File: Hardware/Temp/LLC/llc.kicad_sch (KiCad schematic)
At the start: 23 parts, among them M1 650 V, 24 A, M2 650 V, 24 A, U1 IR2101, U2 OPAMP_OP07CSZ

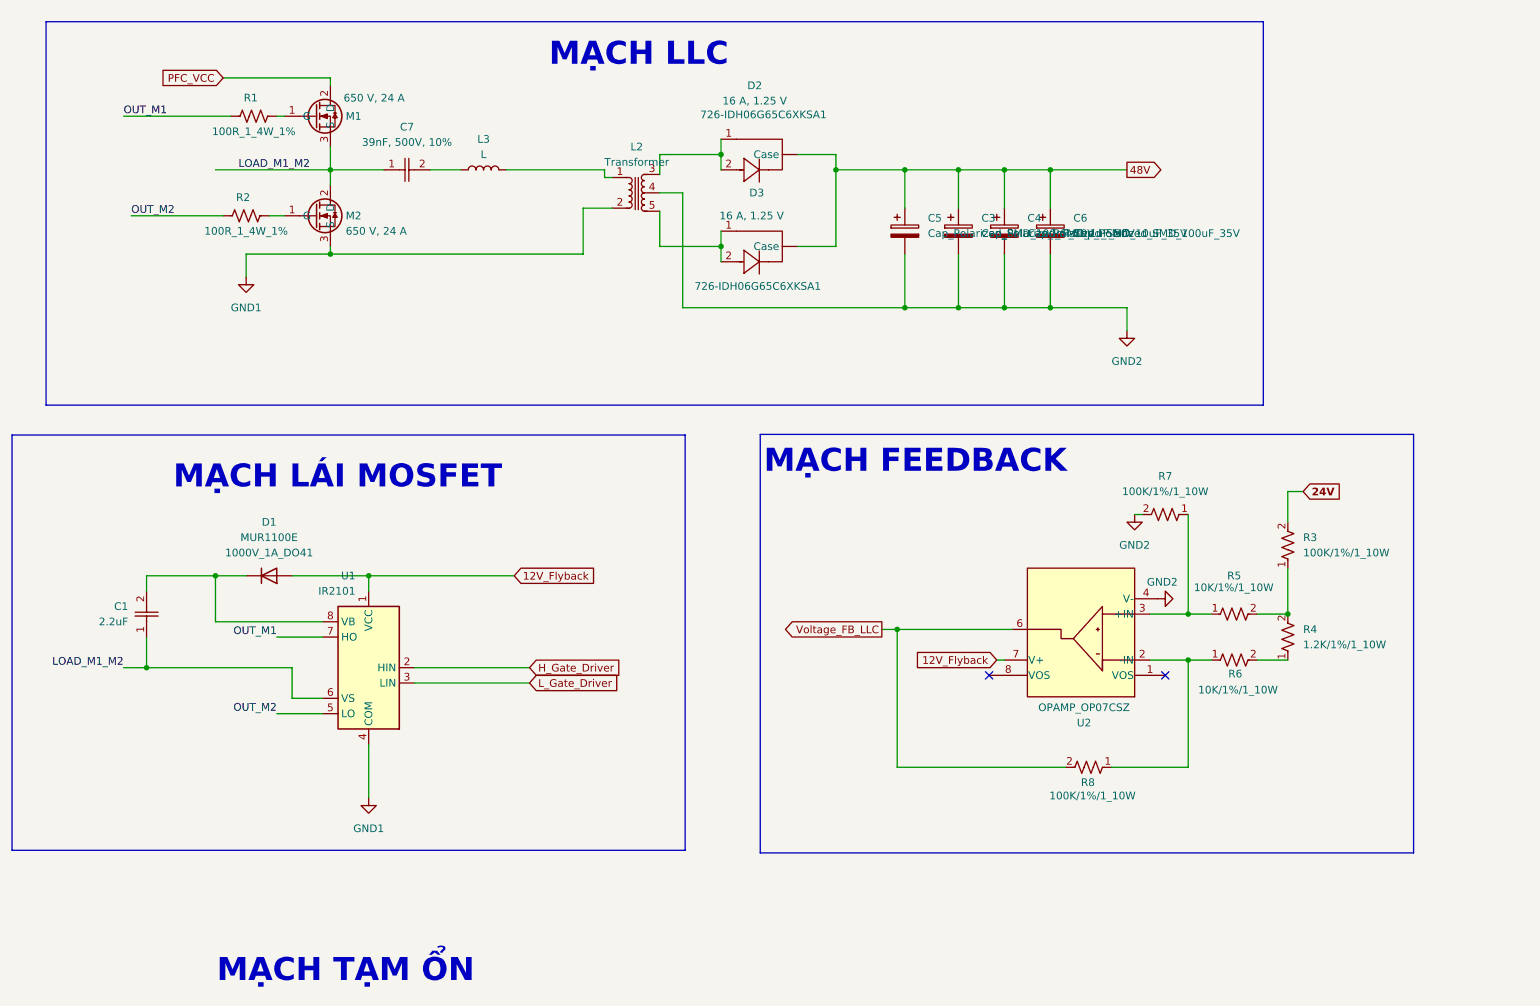
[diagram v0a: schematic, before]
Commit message: hardware:sche: update schematic F4, F1
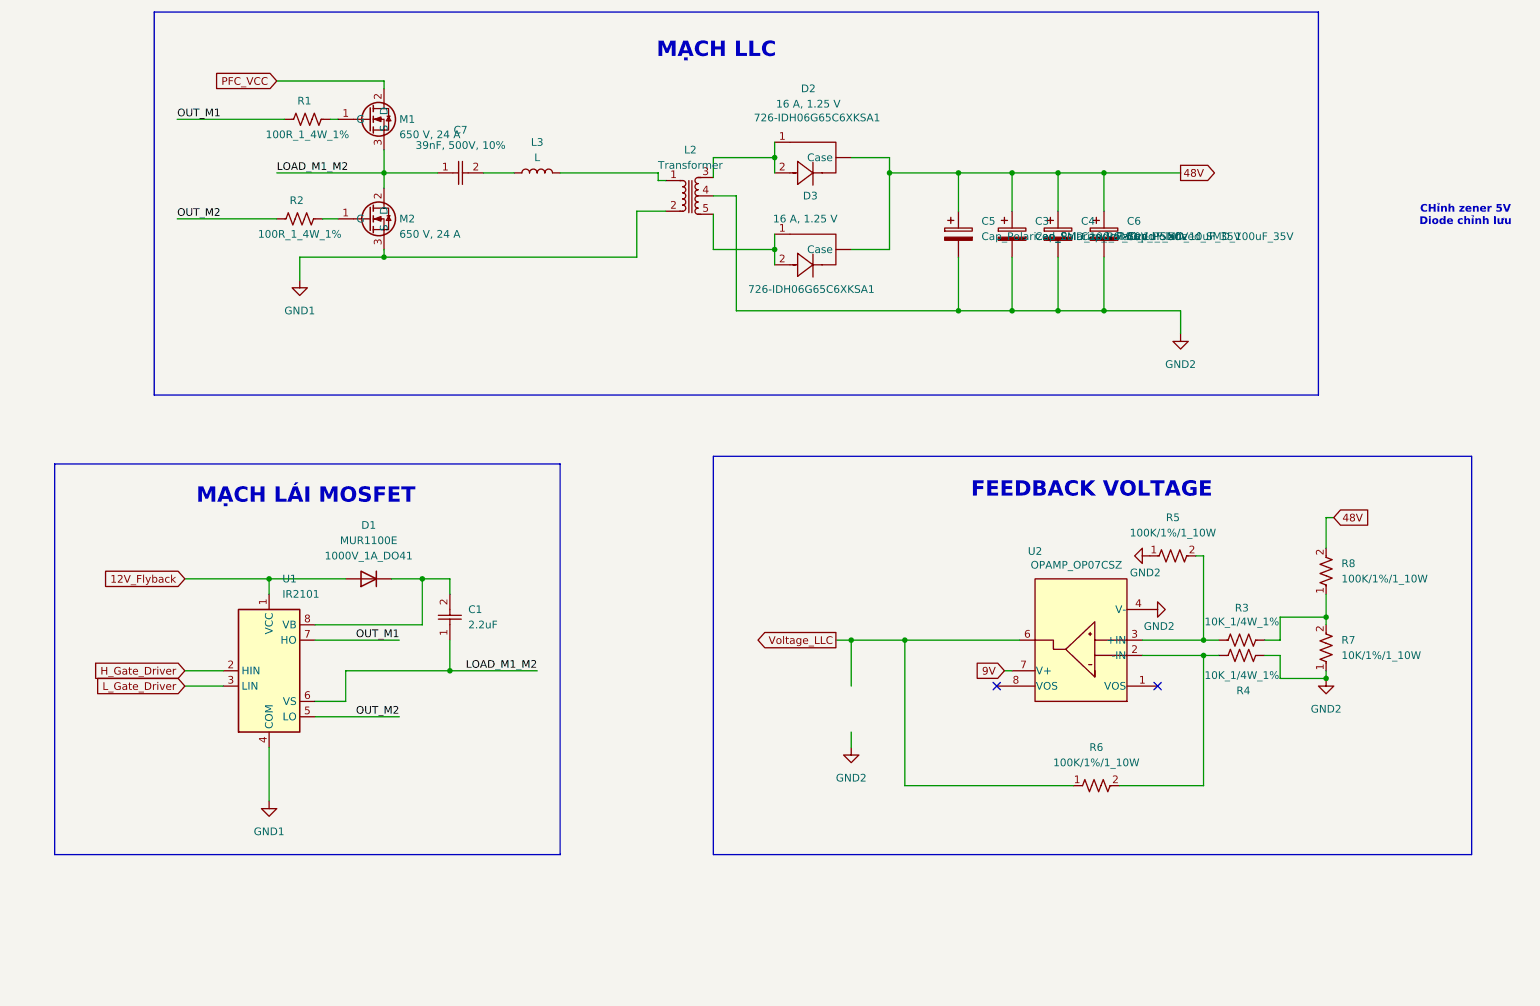
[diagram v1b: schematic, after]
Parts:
- removed R3, R7: 100K/1%/1_10W, charge_battery_footprint_lib:Res_200K_0603, symbol charge_battery_sym_lib:Res_200K_0603_1%
- removed R4: 1.2K/1%/1_10W, charge_battery_footprint_lib:Res_200K_0603, symbol charge_battery_sym_lib:Res_200K_0603_1%
- removed R5, R6: 10K/1%/1_10W, charge_battery_footprint_lib:Res_10K_0603, symbol charge_battery_sym_lib:Res_10K_0603_1%
- added R3, R4: 10K_1/4W_1%, charge_battery_footprint_lib:Res_10K_1_4W_1%, symbol charge_battery_sym_lib:Res_hole_10K_1/4W_1%
- added R5, R6: 100K/1%/1_10W, charge_battery_footprint_lib:Res_200K_0603, symbol charge_battery_sym_lib:Res_200K_0603_1%
- added R7: 10K/1%/1_10W, charge_battery_footprint_lib:Res_10K_0603, symbol charge_battery_sym_lib:Res_10K_0603_1%
- C1: value 2.2uF -> 2.2uF
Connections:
- net 12V_Flyback: no longer U2.7 (V+)
- net 48V: now also R8.2
- net GND2: now also R4.2, R5.1, R7.1
- net at R8.1: now also R3.2, R7.2; no longer U2.2 (-IN)
- net at U2.3 (+IN): now also R3.1, R5.2
- net Voltage_FB_LLC renamed Voltage_LLC
- net Voltage_LLC: now also R6.1; no longer R8.2
- new net: R4.1, R6.2, U2.2 (-IN)
- new net 9V: U2.7 (V+)
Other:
- note added: "CHỉnh zener 5V Diode chỉnh lưu"
- note added: "FEEDBACK VOLTAGE"
- note removed: "MẠCH FEEDBACK"
- note removed: "MẠCH TẠM ỔN"
- moved on the sheet: C1, C3, C4, C5, C6, C7, D1, D2, D3, L2, L3, M1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
